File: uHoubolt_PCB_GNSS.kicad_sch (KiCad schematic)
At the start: 103 parts, among them J1 Power In, J10 CAN1, J11 CAN2, J12 MMCX-J-P-H-ST-SM1, J2 Debug, J3 Debug, J4 CAN1, J5 CAN2, J6 CAN1, J7 CAN2, J8 CAN1, J9 CAN2, Q1 SISA88DN or similar, U1 SAM-M8Q, U10 LoRa1278F30, U11 LPS25HB, U2 STM32G491MET6-LQFP80, U3 W25Q256JV, U4 MCP1700-3302E, U5 MCP2562FDT-H_SN, U6 MCP2562FDT-H_SN, U7 TS30041, U8 MCP1700-3302E, U9 ICM-20602, X1 TXC-7C

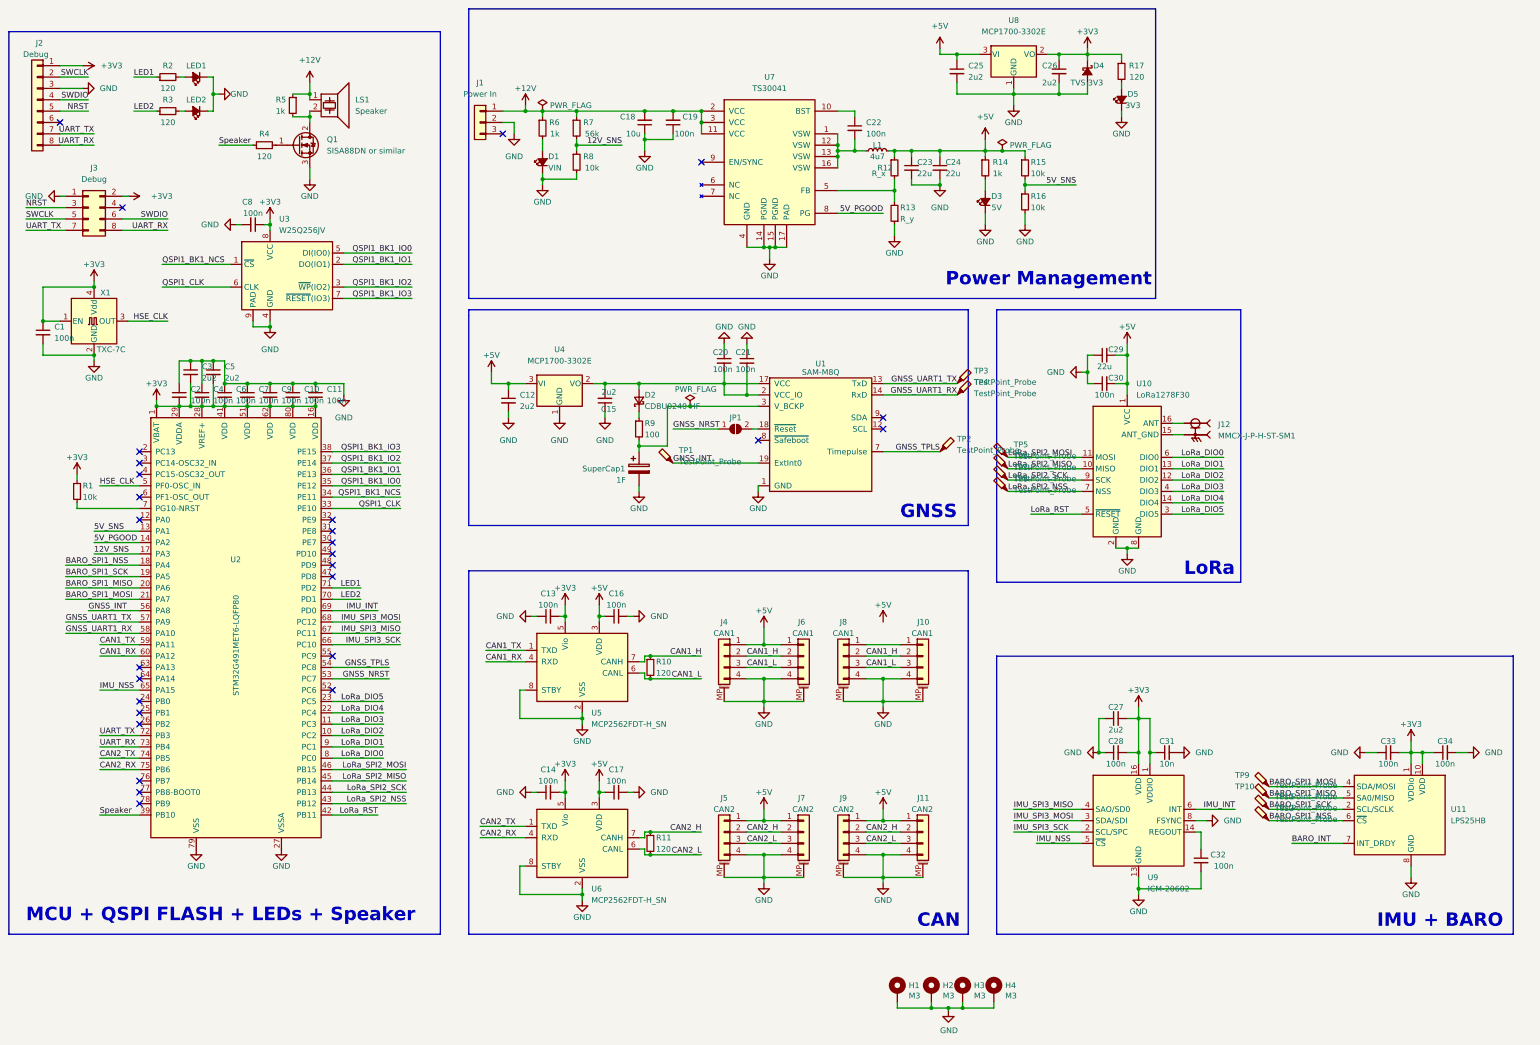
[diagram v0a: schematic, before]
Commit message: Update layout further
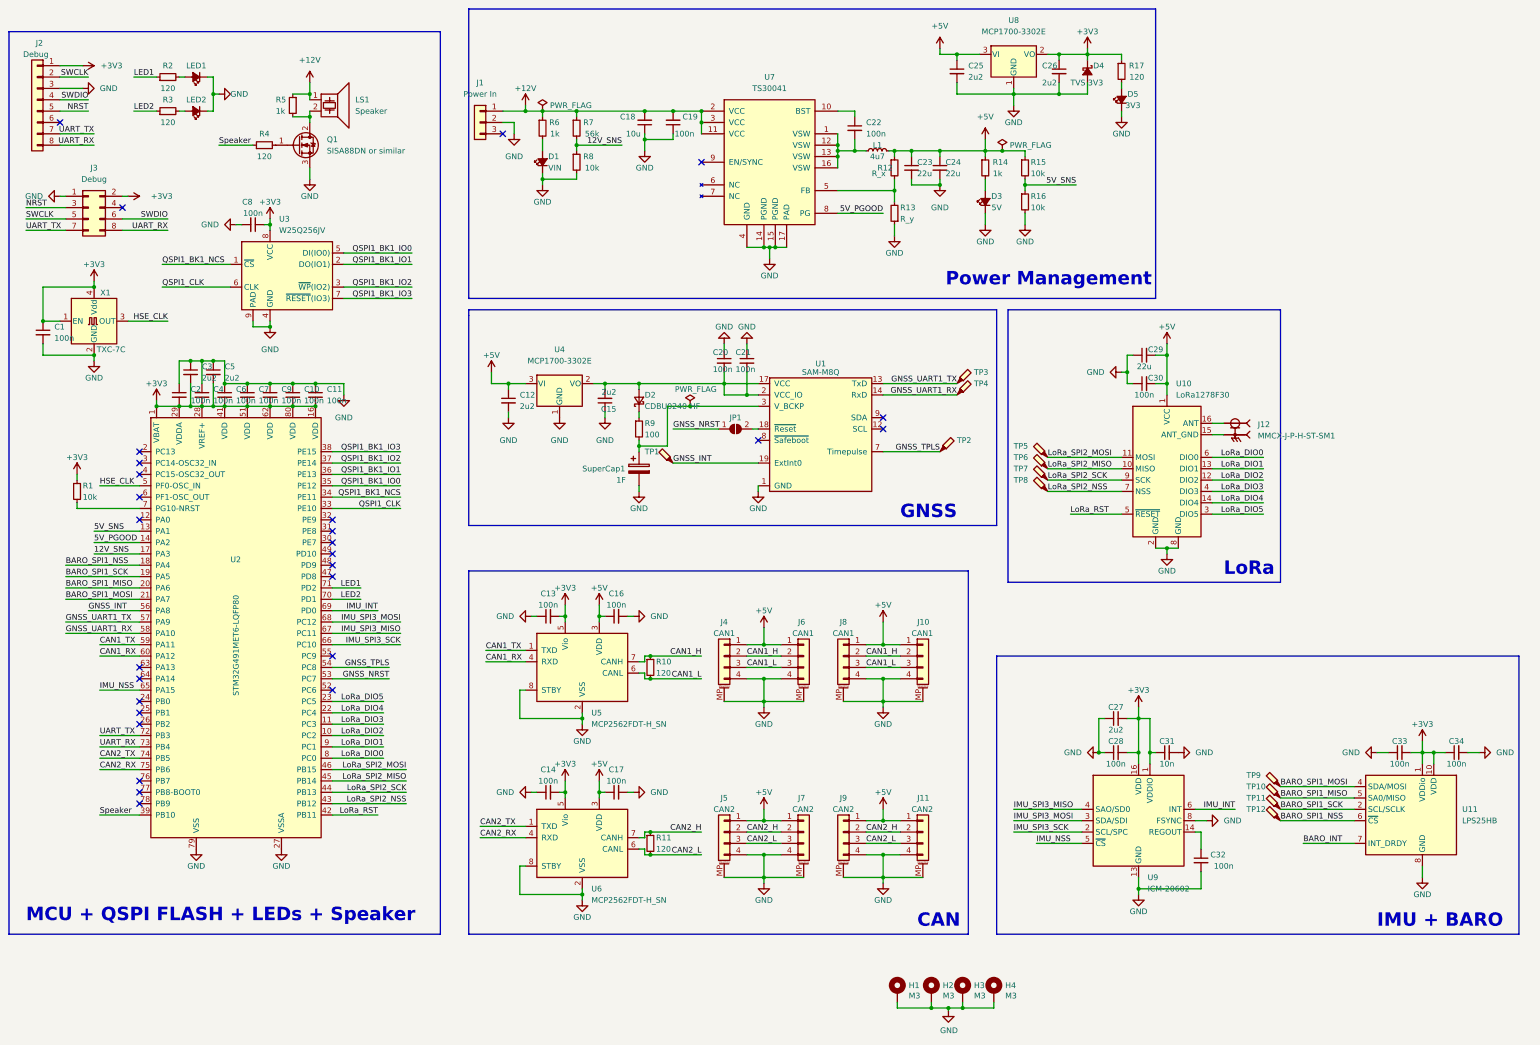
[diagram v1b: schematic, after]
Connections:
- net +5V: now also J10.1 (Pin_1), J8.1 (Pin_1)
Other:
- moved on the sheet: C29, C30, C33, C34, J12, TP10, TP11, TP12, TP5, TP6, TP7, TP8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
